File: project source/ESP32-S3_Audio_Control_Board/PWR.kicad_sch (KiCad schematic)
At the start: 42 parts, among them J19 Barrel_Jack, Q1 DMP3013SFV-7, U2 TPS54331D, U6 TPS54331D

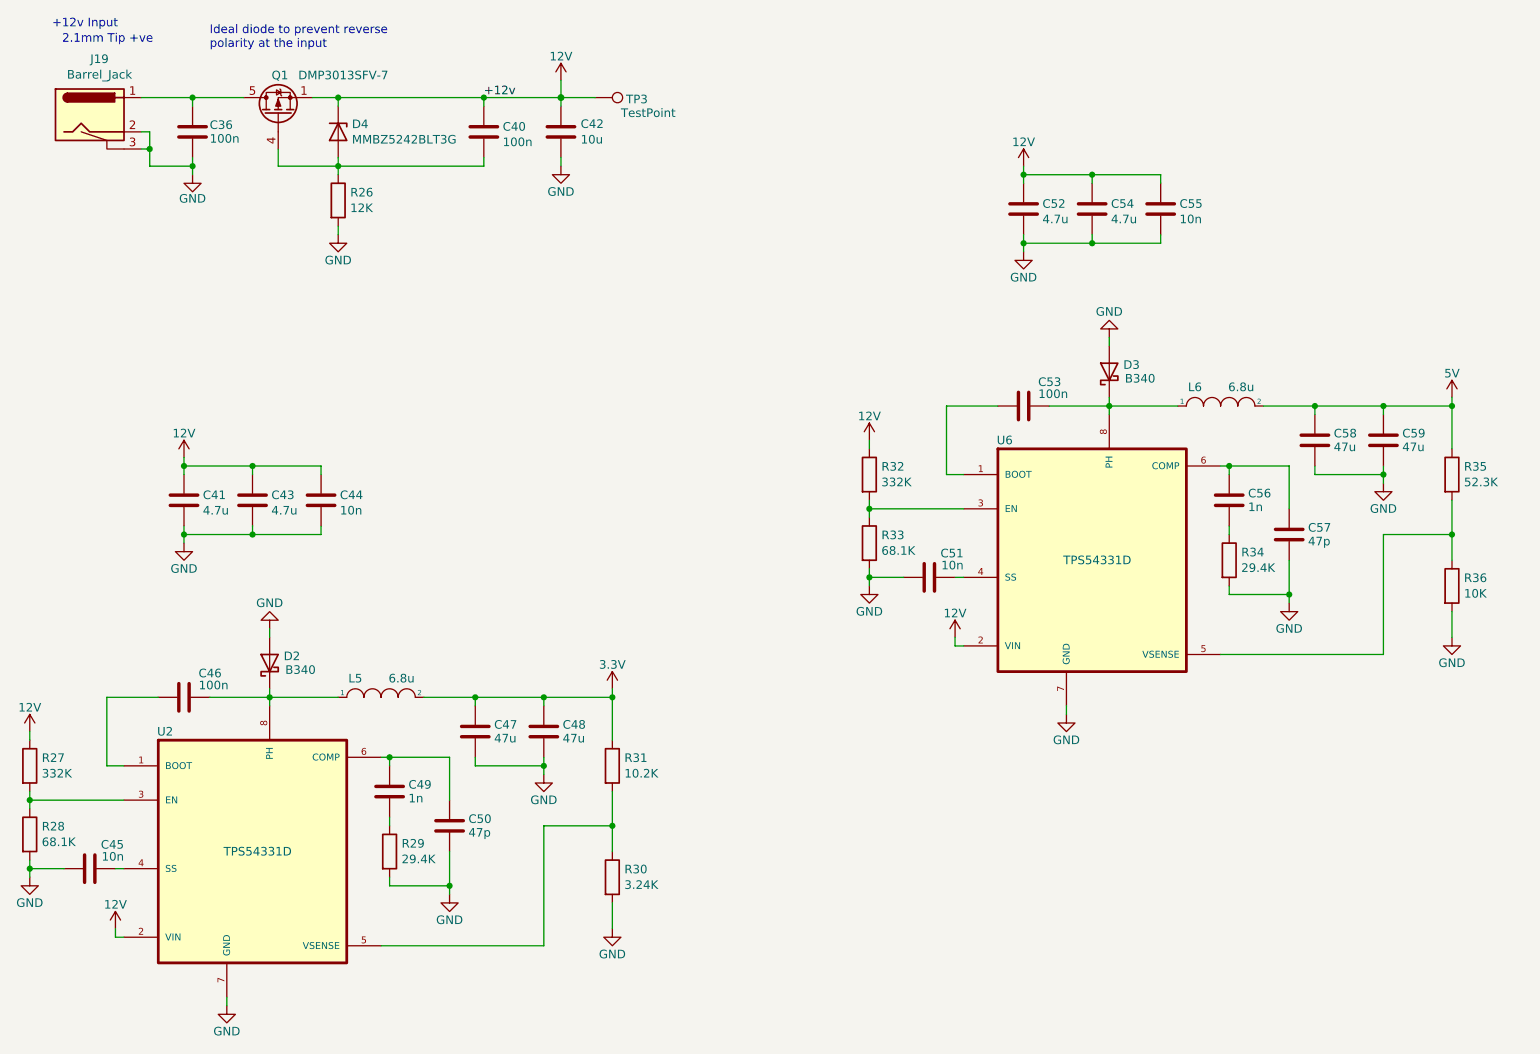
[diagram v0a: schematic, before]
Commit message: update
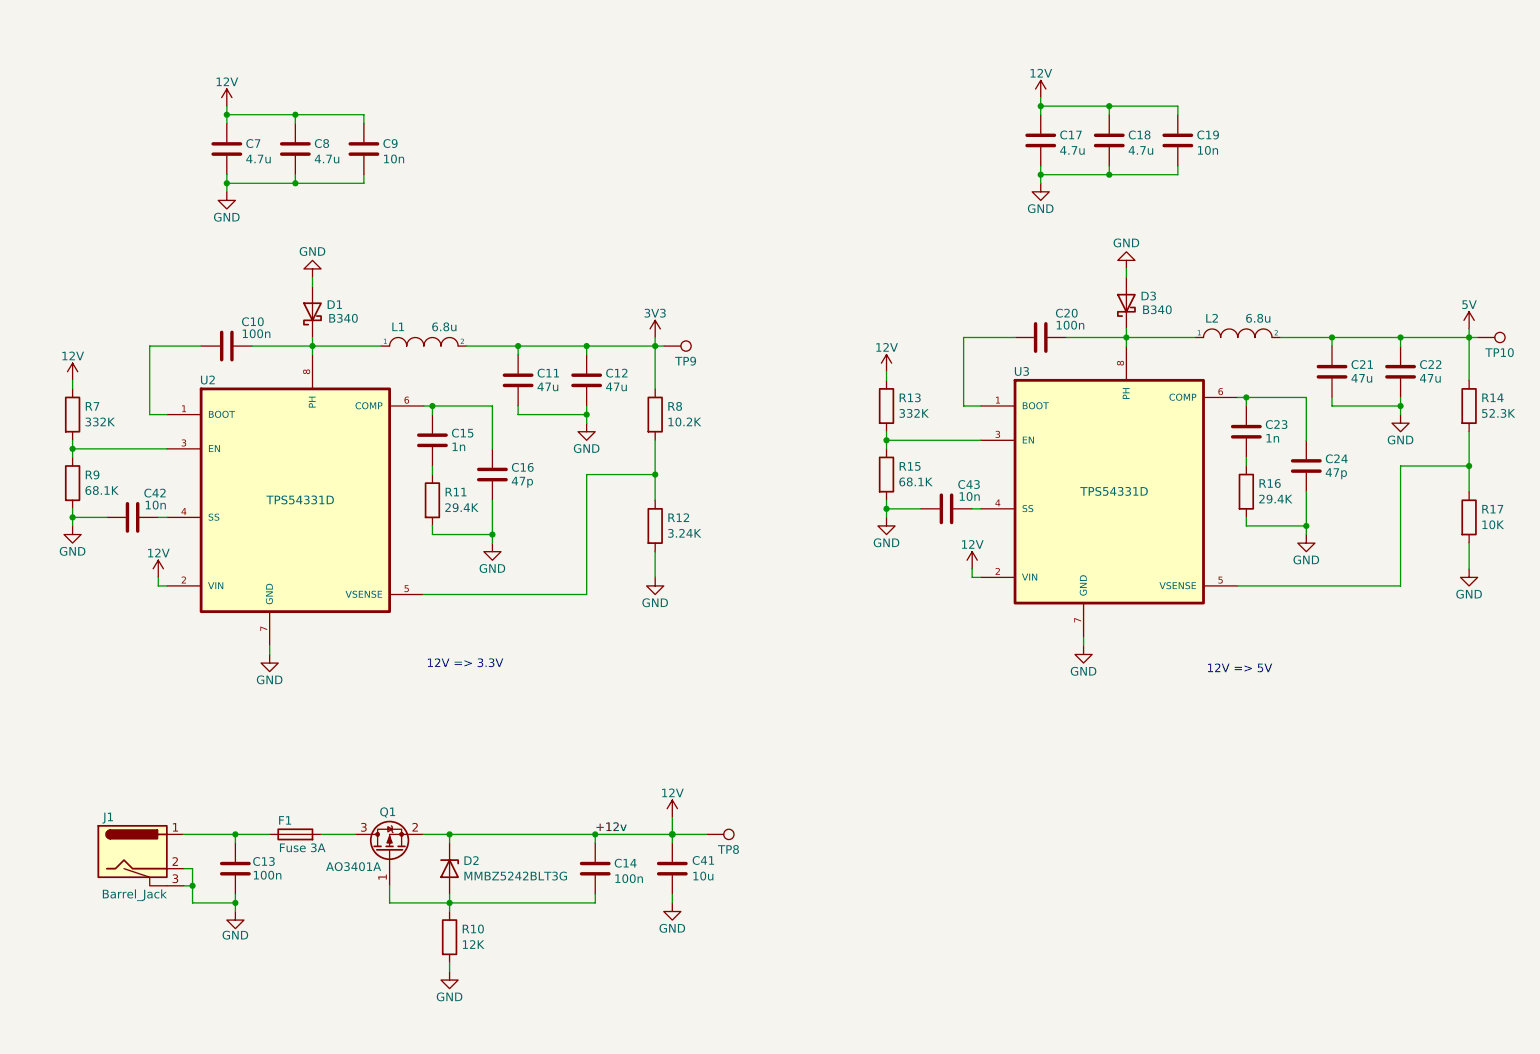
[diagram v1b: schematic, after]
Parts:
- removed L5: 6.8u, Inductor_SMD:L_Bourns_SRP7028A_7.3x6.6mm, symbol pspice:INDUCTOR
- removed Q1: DMP3013SFV-7, Package_SON:Diodes_PowerDI3333-8, symbol Transistor_FET:DMP3013SFV
- removed TP3: TestPoint, TestPoint:TestPoint_Pad_2.0x2.0mm, symbol Connector:TestPoint
- removed U6: TPS54331D, Audio_control_board:TPS54331, symbol TPS54331:TPS54331D
- added F1: Fuse 3A, Resistor_SMD:R_1812_4532Metric, symbol Device:Fuse
- added L1: 6.8u, Inductor_SMD:L_Sunlord_MWSA0602S, symbol pspice:INDUCTOR
- added Q1: AO3401A, Package_TO_SOT_SMD:SOT-23, symbol Transistor_FET:AO3401A
- added TP10, TP8, TP9: IO0, TestPoint:TestPoint_Pad_D1.5mm, symbol Connector:TestPoint
- added U3: TPS54331D, Package_SO:SOIC-8-1EP_3.9x4.9mm_P1.27mm_EP2.29x3mm, symbol TPS54331:TPS54331D
- C11: renamed from C47; footprint 1210 -> Capacitor_SMD:C_1210_3225Metric
- C12: renamed from C48; footprint 1210 -> Capacitor_SMD:C_1210_3225Metric
- C14: renamed from C40; Field4 Farnell -> (none); Field5 2611911 -> (none); Field6 RM EMK105 B7104KV-F -> (none); Field7 TAIYO YUDEN EUROPE GMBH -> (none); Field8 110091611 -> (none); Mfr (none) -> Murata Electronics; Mfr PN (none) -> GRM155R71H104KE14D; Part Description 0.1uF 10% 16V Ceramic Capacitor X7R 0402 (1005 Metric) -> 100nF 50V X7R ±10% 0402 Multilayer Ceramic Capacitors MLCC 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; Supplier (none) -> RM EMK105 B7104KV-F; Supplier PN (none) -> C77020
- C15: renamed from C49; footprint 0402 -> Capacitor_SMD:C_0402_1005Metric
- C16: renamed from C50; footprint 0402 -> Capacitor_SMD:C_0402_1005Metric
- C21: renamed from C58; footprint 1210 -> Capacitor_SMD:C_1210_3225Metric
- C22: renamed from C59; footprint 1210 -> Capacitor_SMD:C_1210_3225Metric
- C23: renamed from C56; footprint 0402 -> Capacitor_SMD:C_0402_1005Metric
- C24: renamed from C57; footprint 0402 -> Capacitor_SMD:C_0402_1005Metric
- C41: renamed from C42; Field4 Digikey -> (none); Field5 490-10505-1-ND -> (none); Field6 GRM21BC8YA106KE11L -> (none); Field7 Murata -> (none); Mfr (none) -> Murata Electronics; Mfr PN (none) -> GRM21BR6YA106KE43L; Part Description 10uF 10% or 20% 35V Ceramic Capacitor X6S 0805 (2012 Metric) -> 10uF 35V X5R ±10% 0805 Multilayer Ceramic Capacitors MLCC -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; Supplier (none) -> LCSC; Supplier PN (none) -> C162422
- D2: renamed from D4; footprint Diode_SMD:D_SOT-23_ANK -> Package_TO_SOT_SMD:TSOT-23; Field4 Digikey -> (none); Field5 MMBZ5242BLT3GOSCT-ND -> (none); Field6 MMBZ5242BLT3G -> (none); Field7 Onsemi -> (none); Mfr (none) -> onsemi; Mfr PN (none) -> MMBZ5242BLT3G; Supplier (none) -> LCSC; Supplier PN (none) -> C896784
- J1: renamed from J19; Field4 Toby -> (none); Field5 DC-001-A-2.1mm-R -> (none); Field6 DC-001-A-2.1mm-R -> (none); Field7 Valcon -> (none); Mfr (none) -> CUI; Mfr PN (none) -> PJ-102AH; Supplier (none) -> LCSC; Supplier PN (none) -> C3096093
- L2: renamed from L6; footprint Inductor_SMD:L_Bourns_SRP7028A_7.3x6.6mm -> Inductor_SMD:L_Sunlord_MWSA0602S
- R10: renamed from R26; Field4 Farnell -> (none); Field5 9239367 -> (none); Field6 MCR01MZPF1202 -> (none); Field7 Rohm -> (none); Mar (none) -> UNI-ROYAL(Uniroyal Elec); Mfr PN (none) -> 0402WGF1202TCE; Part Description Resistor 12K M1005 1% 63mW -> -55℃~+155℃ 12kΩ 50V 62.5mW Thick Film Resistor ±1% ±100ppm/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; Supplier (none) -> LCSC; Supplier PN (none) -> C25752
- U2: footprint Audio_control_board:TPS54331 -> Package_SO:SOIC-8-1EP_3.9x4.9mm_P1.27mm_EP2.29x3mm; Availability In Stock -> (none); Check_prices https://www.snapeda.com/parts/TPS54331D/Texas+Instruments/v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 -> (none); MF Texas Instruments -> (none); MP TPS54331D -> (none); Mfr (none) -> Texas Instruments; Mfr PN (none) -> TPS54331DR; Package SOIC-8 Texas Instruments -> (none); Part Description (none) -> -40℃~+150℃@(TJ) 1 110uA 3.5V~28V 3A 570kHz 800mV~25V Adjust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; Price None -> (none); SnapEDA_Link https://www.snapeda.com/parts/TPS54331D/Texas+Instruments/v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 -> (none); Supplier (none) -> LCSC; Supplier PN (none) -> C9865
- renumbered C46 to C10, C36 to C13, C52 to C17, C54 to C18, C55 to C19, C53 to C20, C45 to C42, C51 to C43, C41 to C7, C43 to C8, C44 to C9, D2 to D1, R29 to R11, R30 to R12, R32 to R13, R35 to R14, R33 to R15, R34 to R16, R36 to R17, R27 to R7, R31 to R8, R28 to R9
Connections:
- net 12V: now also Q1.2 (S), TP8.1, U3.2 (VIN)
- net 5V: now also TP10.1
- net GND: now also U3.7 (GND)
- net at C14.2, D2.2 (A), R10.1: now also Q1.1 (G)
- net at C43.2: now also U3.4 (SS)
- net at R13.2, R15.1: now also U3.3 (EN)
- net at C10.2, D1.1 (K), U2.8 (PH): now also L1.1
- net at C20.2, D3.1 (K), L2.1: now also U3.8 (PH)
- net at C20.1: now also U3.1 (BOOT)
- net at R14.2, R17.1: now also U3.5 (VSENSE)
- net at C23.2, C24.2: now also U3.6 (COMP)
- net at C13.1, J1.1: now also F1.1
- net 3.3V renamed 3V3
- net 3V3: now also L1.2, TP9.1
- new net: F1.2, Q1.3 (D)
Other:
- note added: "12V => 3.3V"
- note added: "12V => 5V"
- note removed: "+12v Input"
- note removed: "2.1mm Tip +ve"
- note removed: "Ideal diode to prevent reverse polarity at the input"
- moved on the sheet: C10, C11, C12, C13, C14, C15, C16, C17, C18, C19, C20, C21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
